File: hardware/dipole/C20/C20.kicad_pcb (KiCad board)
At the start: 2 copper layers, 110 x 60 mm, 2 parts, among them J1 Conn_01x01, J2 Conn_01x01

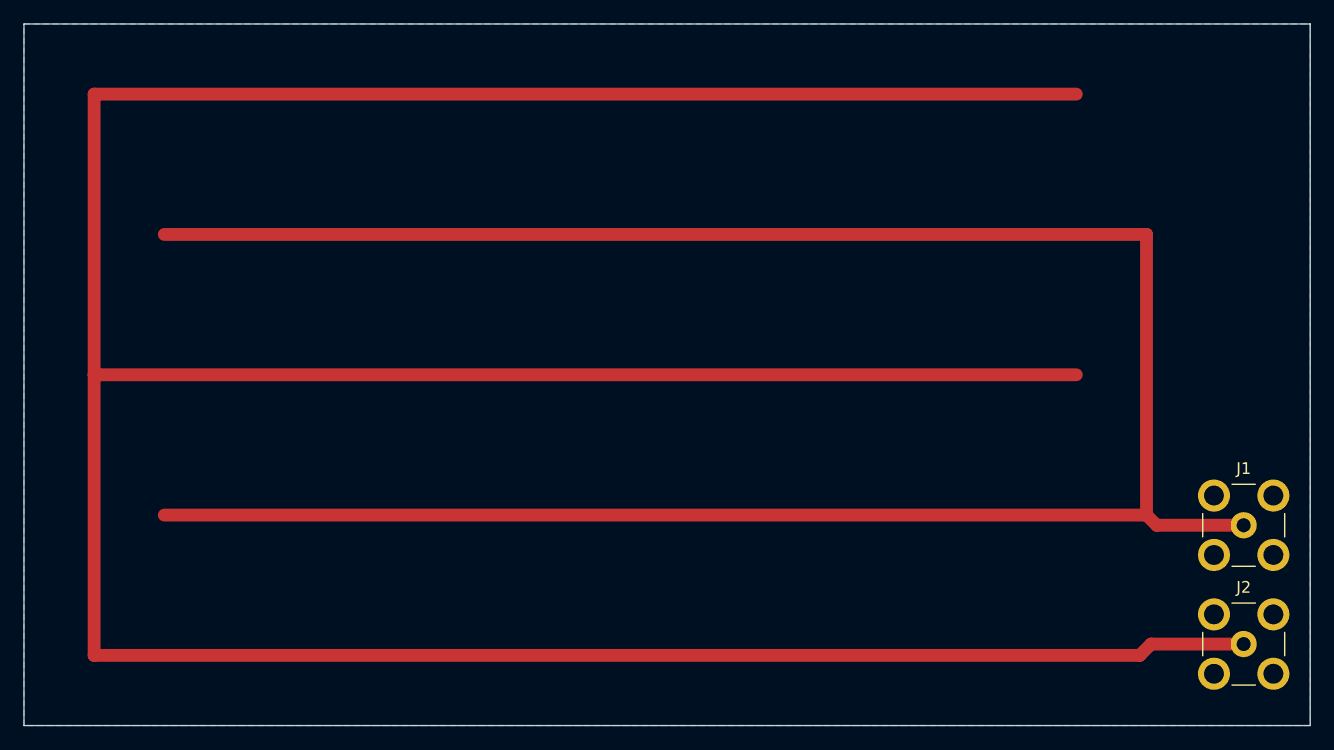
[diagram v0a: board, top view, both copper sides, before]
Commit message: add  analysis conception and simulation part of the rapport
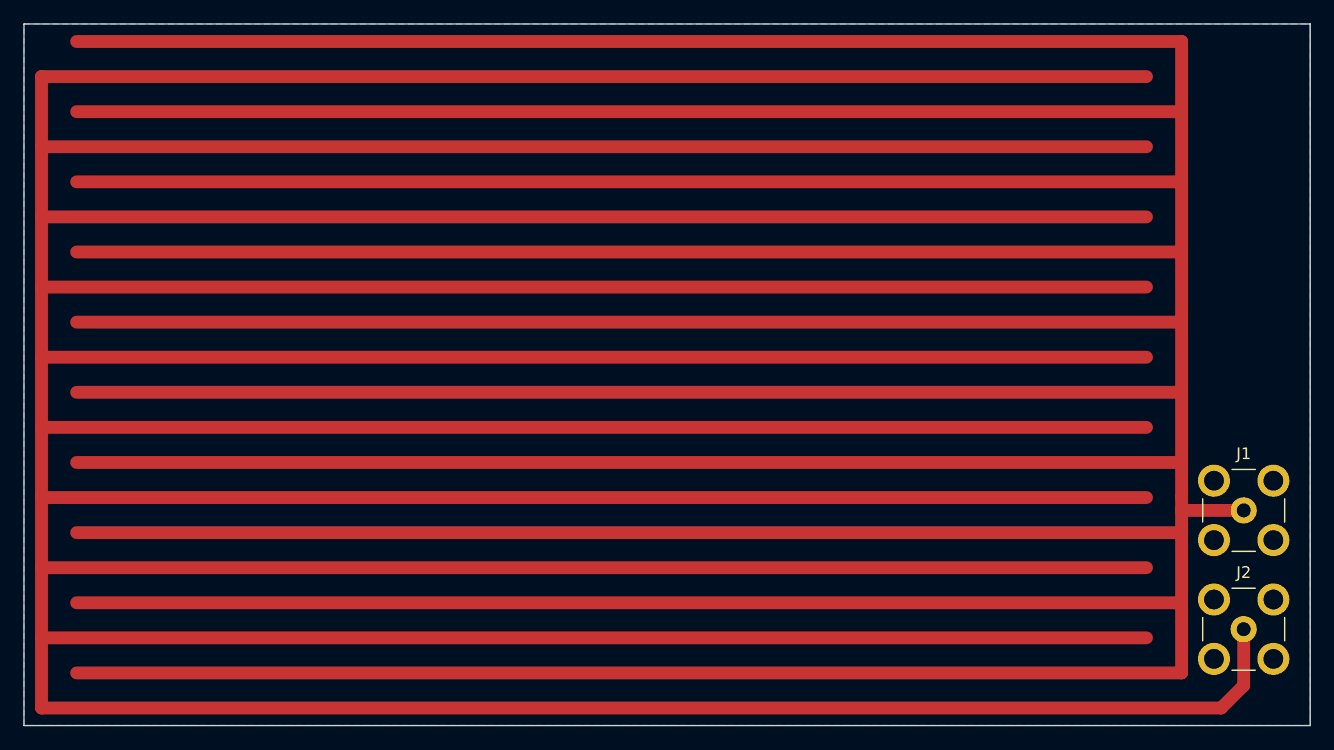
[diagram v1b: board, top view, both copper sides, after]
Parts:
- moved J1 1.27 mm to (194.3, 101.6)
- moved J2 1.27 mm to (194.3, 111.8)
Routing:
- net unconnected-(J1-Pin_1-Pad1): track 200.7 -> 1004.3 mm
- net unconnected-(J2-Pin_1-Pad1): track 314.7 -> 1012.9 mm
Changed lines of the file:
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@@
   (net 2 "unconnected-(J2-Pin_1-Pad1)")
   (footprint "Connector_Coaxial:SMB_Jack_Vertical" (layer "F.Cu")
-    (at 194.31 102.87)
+    (at 194.31 101.6)
     (descr "SMB pcb mounting jack")
     (tags "SMB Jack  Striaght")
@@
   )
   (footprint "Connector_Coaxial:SMB_Jack_Vertical" (layer "F.Cu")
-    (at 194.31 113.03)
+    (at 194.31 111.76)
     (descr "SMB pcb mounting jack")
     (tags "SMB Jack  Striaght")
@@
   (gr_rect (start 90 60) (end 200 120)
     (stroke (width 0.1) (type default)) (fill none) (layer "Edge.Cuts"))
-  (segment (start 186 102) (end 102 102) (width 1.1) (layer "F.Cu") (net 1))
-  (segment (start 186.87 102.87) (end 186 102) (width 1.1) (layer "F.Cu") (net 1))
-  (segment (start 102 78) (end 186 78) (width 1.1) (layer "F.Cu") (net 1))
-  (segment (start 194.31 102.87) (end 186.87 102.87) (width 1.1) (layer "F.Cu") (net 1))
-  (segment (start 186 78) (end 186 102) (width 1.1) (layer "F.Cu") (net 1))
-  (segment (start 96 90) (end 180 90) (width 1.1) (layer "F.Cu") (net 2))
-  (segment (start 185.42 114) (end 96 114) (width 1.1) (layer "F.Cu") (net 2))
-  (segment (start 96 66) (end 96 90) (width 1.1) (layer "F.Cu") (net 2))
-  (segment (start 185.42 114) (end 186.39 113.03) (width 1.1) (layer "F.Cu") (net 2))
-  (segment (start 186.39 113.03) (end 194.31 113.03) (width 1.1) (layer "F.Cu") (net 2))
-  (segment (start 96 114) (end 96 90) (width 1.1) (layer "F.Cu") (net 2))
-  (segment (start 180 66) (end 96 66) (width 1.1) (layer "F.Cu") (net 2))
+  (segment (start 189 61.5) (end 189 67.5) (width 1.1) (layer "F.Cu") (net 1))
+  (segment (start 189 73.5) (end 189 79.5) (width 1.1) (layer "F.Cu") (net 1))
+  (segment (start 94.5 67.5) (end 189 67.5) (width 1.1) (layer "F.Cu") (net 1))
+  (segment (start 189 79.5) (end 189 85.5) (width 1.1) (layer "F.Cu") (net 1))
+  (segment (start 189 97.5) (end 189 100.5) (width 1.1) (layer "F.Cu") (net 1))
+  (segment (start 189 103.5) (end 189 109.5) (width 1.1) (layer "F.Cu") (net 1))
+  (segment (start 94.5 61.5) (end 189 61.5) (width 1.1) (layer "F.Cu") (net 1))
+  (segment (start 94.5 109.5) (end 189 109.5) (width 1.1) (layer "F.Cu") (net 1))
+  (segment (start 94.5 103.5) (end 189 103.5) (width 1.1) (layer "F.Cu") (net 1))
+  (segment (start 189 101.6) (end 189 103.5) (width 1.1) (layer "F.Cu") (net 1))
+  (segment (start 194.31 101.6) (end 189 101.6) (width 1.1) (layer "F.Cu") (net 1))
+  (segment (start 94.5 91.5) (end 189 91.5) (width 1.1) (layer "F.Cu") (net 1))
+  (segment (start 189 100.5) (end 189 101.6) (width 1.1) (layer "F.Cu") (net 1))
+  (segment (start 189 85.5) (end 189 91.5) (width 1.1) (layer "F.Cu") (net 1))
+  (segment (start 94.5 97.5) (end 189 97.5) (width 1.1) (layer "F.Cu") (net 1))
+  (segment (start 189 109.5) (end 189 115.5) (width 1.1) (layer "F.Cu") (net 1))
+  (segment (start 94.5 85.5) (end 189 85.5) (width 1.1) (layer "F.Cu") (net 1))
+  (segment (start 189 115.5) (end 94.5 115.5) (width 1.1) (layer "F.Cu") (net 1))
+  (segment (start 94.5 73.5) (end 189 73.5) (width 1.1) (layer "F.Cu") (net 1))
+  (segment (start 189 91.5) (end 189 97.5) (width 1.1) (layer "F.Cu") (net 1))
+  (segment (start 94.5 79.5) (end 189 79.5) (width 1.1) (layer "F.Cu") (net 1))
+  (segment (start 189 67.5) (end 189 73.5) (width 1.1) (layer "F.Cu") (net 1))
+  (segment (start 91.5 94.5) (end 91.5 88.5) (width 1.1) (layer "F.Cu") (net 2))
+  (segment (start 186 112.5) (end 91.5 112.5) (width 1.1) (layer "F.Cu") (net 2))
+  (segment (start 91.5 76.5) (end 91.5 70.5) (width 1.1) (layer "F.Cu") (net 2))
+  (segment (start 192.39 118.5) (end 91.5 118.5) (width 1.1) (layer "F.Cu") (net 2))
+  (segment (start 91.5 88.5) (end 91.5 82.5) (width 1.1) (layer "F.Cu") (net 2))
+  (segment (start 91.5 64.5) (end 186 64.5) (width 1.1) (layer "F.Cu") (net 2))
+  (segment (start 186 70.5) (end 91.5 70.5) (width 1.1) (layer "F.Cu") (net 2))
+  (segment (start 194.31 111.76) (end 194.31 116.58) (width 1.1) (layer "F.Cu") (net 2))
+  (segment (start 186 94.5) (end 91.5 94.5) (width 1.1) (layer "F.Cu") (net 2))
+  (segment (start 91.5 100.5) (end 91.5 94.5) (width 1.1) (layer "F.Cu") (net 2))
+  (segment (start 186 76.5) (end 91.5 76.5) (width 1.1) (layer "F.Cu") (net 2))
+  (segment (start 91.5 106.5) (end 91.5 100.5) (width 1.1) (layer "F.Cu") (net 2))
+  (segment (start 91.5 70.5) (end 91.5 64.5) (width 1.1) (layer "F.Cu") (net 2))
+  (segment (start 91.5 82.5) (end 91.5 76.5) (width 1.1) (layer "F.Cu") (net 2))
+  (segment (start 186 82.5) (end 91.5 82.5) (width 1.1) (layer "F.Cu") (net 2))
+  (segment (start 91.5 118.5) (end 91.5 112.5) (width 1.1) (layer "F.Cu") (net 2))
+  (segment (start 186 106.5) (end 91.5 106.5) (width 1.1) (layer "F.Cu") (net 2))
+  (segment (start 186 100.5) (end 91.5 100.5) (width 1.1) (layer "F.Cu") (net 2))
+  (segment (start 91.5 112.5) (end 91.5 106.5) (width 1.1) (layer "F.Cu") (net 2))
+  (segment (start 194.31 116.58) (end 192.39 118.5) (width 1.1) (layer "F.Cu") (net 2))
+  (segment (start 186 88.5) (end 91.5 88.5) (width 1.1) (layer "F.Cu") (net 2))
   (zone (net 0) (net_name "") (layer "B.Cu") (hatch edge 0.5)
     (connect_pads (clearance 0.5))
